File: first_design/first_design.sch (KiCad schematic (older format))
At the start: 44 parts, among them IC1 BD48K60, IC2 AZ2085, IC3 AP65450, IC4 RN, IC5 VNH7070BAS, J1 Conn_02x20_Odd_Even, J2 Accelerometer_small, J3 Accelerometer_standard, J4 Servo_motor

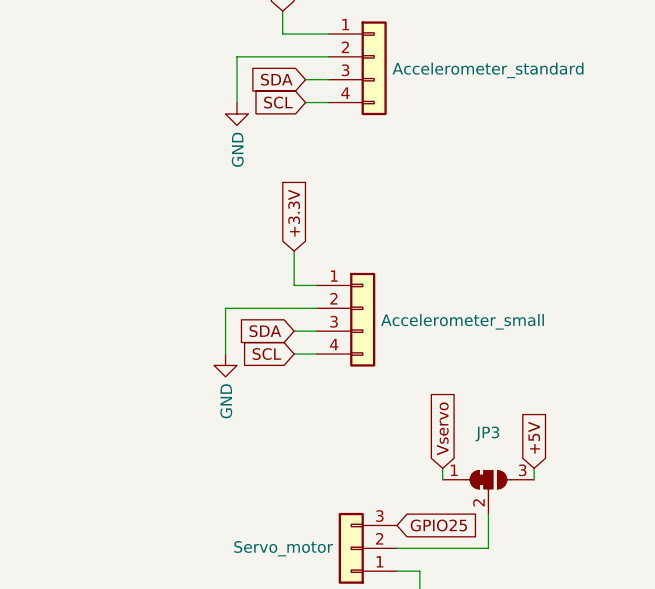
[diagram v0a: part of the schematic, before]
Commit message: final touches
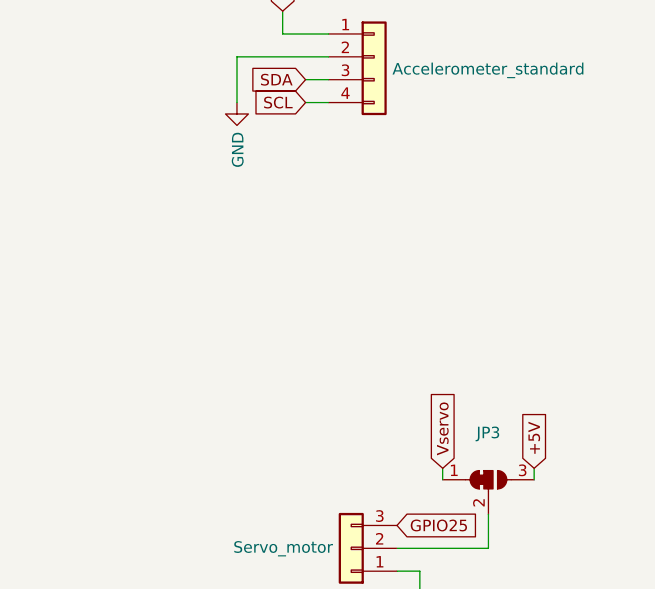
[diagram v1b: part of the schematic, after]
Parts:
- removed J2: Accelerometer_small, library_express_pro:accelerometer_small, symbol Connector_Generic:Conn_01x04
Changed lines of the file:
@@
 $EndComp
-$Comp
-L Connector_Generic:Conn_01x04 J2
-U 1 1 5D5211C9
-P 10000 3700
-F 0 "J2" H 10080 3692 50  0001 L CNN
-F 1 "Accelerometer_small" H 10080 3646 50  0000 L CNN
-F 2 "library_express_pro:accelerometer_small" H 10000 3700 50  0001 C CNN
-F 3 "~" H 10000 3700 50  0001 C CNN
-	1    10000 3700
-	1    0    0    -1
-$EndComp
-Wire Wire Line
-	9800 3600 9700 3600
-Wire Wire Line
-	9800 3800 9700 3800
-Wire Wire Line
-	9800 3900 9700 3900
 $Comp
 L Connector_Generic:Conn_01x04 J3
@@
 Wire Wire Line
 	7500 4400 7550 4400
-Text GLabel 9700 3450 1    50   Input ~ 0
-+3.3V
-$Comp
-L power:GND #PWR0122
-U 1 1 5D60AB58
-P 9400 3900
-F 0 "#PWR0122" H 9400 3650 50  0001 C CNN
-F 1 "GND" V 9405 3772 50  0000 R CNN
-F 2 "" H 9400 3900 50  0001 C CNN
-F 3 "" H 9400 3900 50  0001 C CNN
-	1    9400 3900
-	1    0    0    -1
-$EndComp
-Wire Wire Line
-	9400 3700 9800 3700
-Text GLabel 9700 3800 0    50   Input ~ 0
-SDA
-Text GLabel 9700 3900 0    50   Input ~ 0
-SCL
 Text GLabel 9650 2400 1    50   Input ~ 0
 +3.3V
@@
 	9450 2600 9450 2800
 Wire Wire Line
-	9400 3700 9400 3900
-Wire Wire Line
 	9650 2400 9650 2500
 Wire Wire Line
 	9650 2500 9850 2500
 Wire Wire Line
-	9700 3450 9700 3600
-Wire Wire Line
 	7500 2500 7500 2350
